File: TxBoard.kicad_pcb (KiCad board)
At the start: 2 copper layers, 94 x 31.8 mm, 21 parts, among them J1 RCA Socket, Q1 RU1J002YNTCL, SW1 Pull-Up, SW2 Input(Hi-Z)/Output, SW3 High/Low

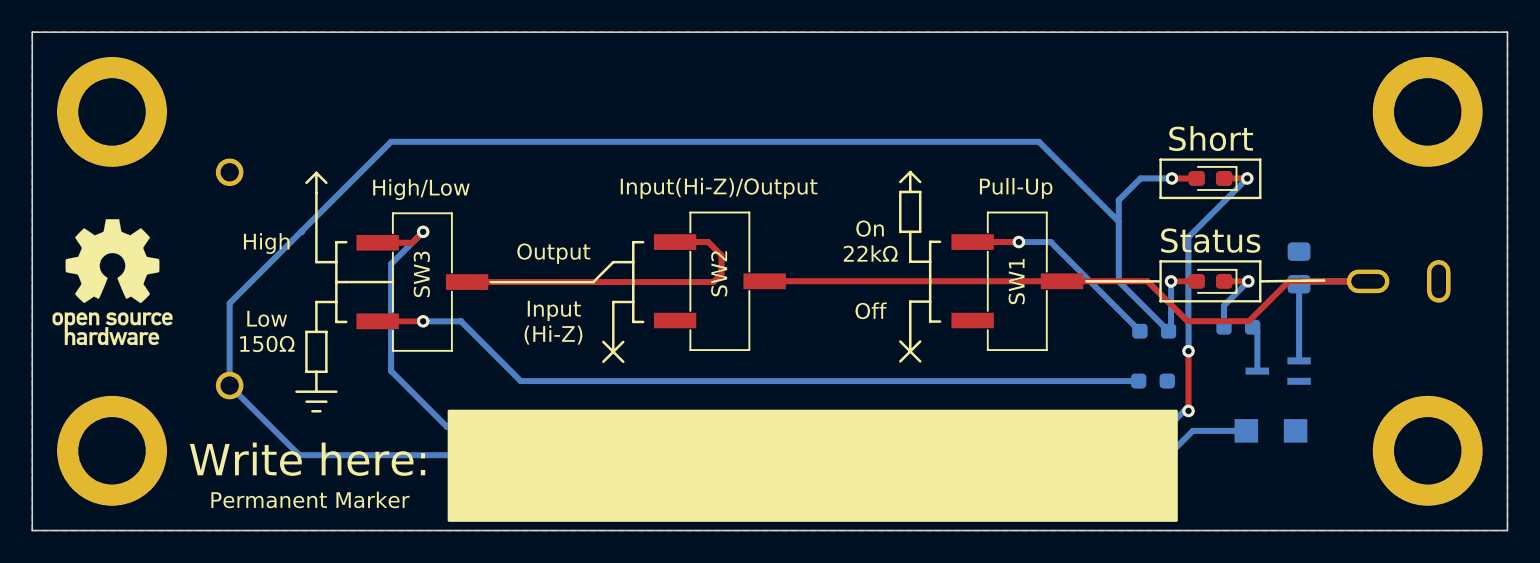
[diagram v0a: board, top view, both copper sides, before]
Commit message: Design review 2
good 4 prototype 2
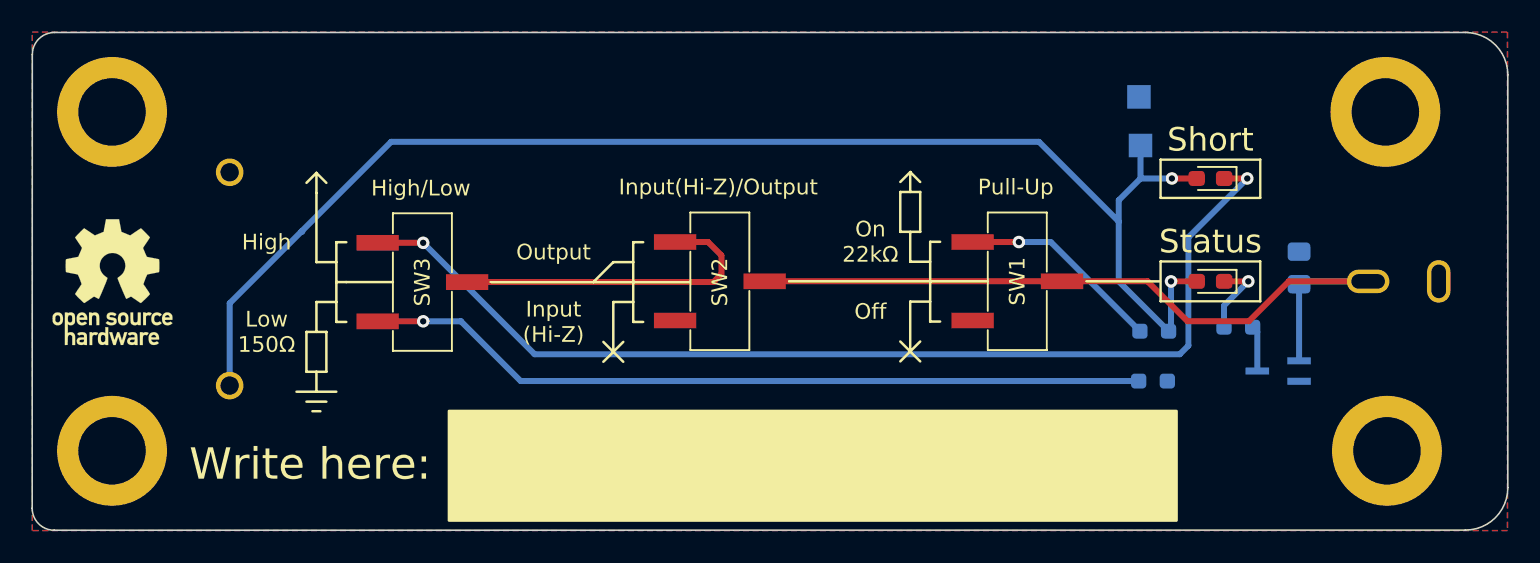
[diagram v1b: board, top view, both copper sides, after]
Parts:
- moved TP1 23.5 mm to (173.5, 85.4)
- moved TP2 19.4 mm to (173.6, 88.5)
- moved REF** 2.70 mm to (189.2, 86.4)
- moved REF** 2.60 mm to (189.3, 108.0)
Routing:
- net +BATT: track 155.7 -> 90.6 mm
- net Net-(SW3-Pad1): track 83.4 -> 68.5 mm, vias 4 -> 2
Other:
- board size 94 x 31.8 mm -> 94 x 31.7 mm
- board text added: "Revision 2 5/7/22"
- board text removed: "Permanent Marker"
- board text removed: "Revision 1 4/19/22"
